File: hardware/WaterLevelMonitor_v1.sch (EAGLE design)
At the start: 38 parts, among them J1 D24V5F5, J2 AVR_SPI_PRG_6PTH, J5 D24V5F5, J6 D24V5F5, J7 RJ45, Q1 NDP6020P, Q4 2N3904, U1 ATMEGA328P_PDIP

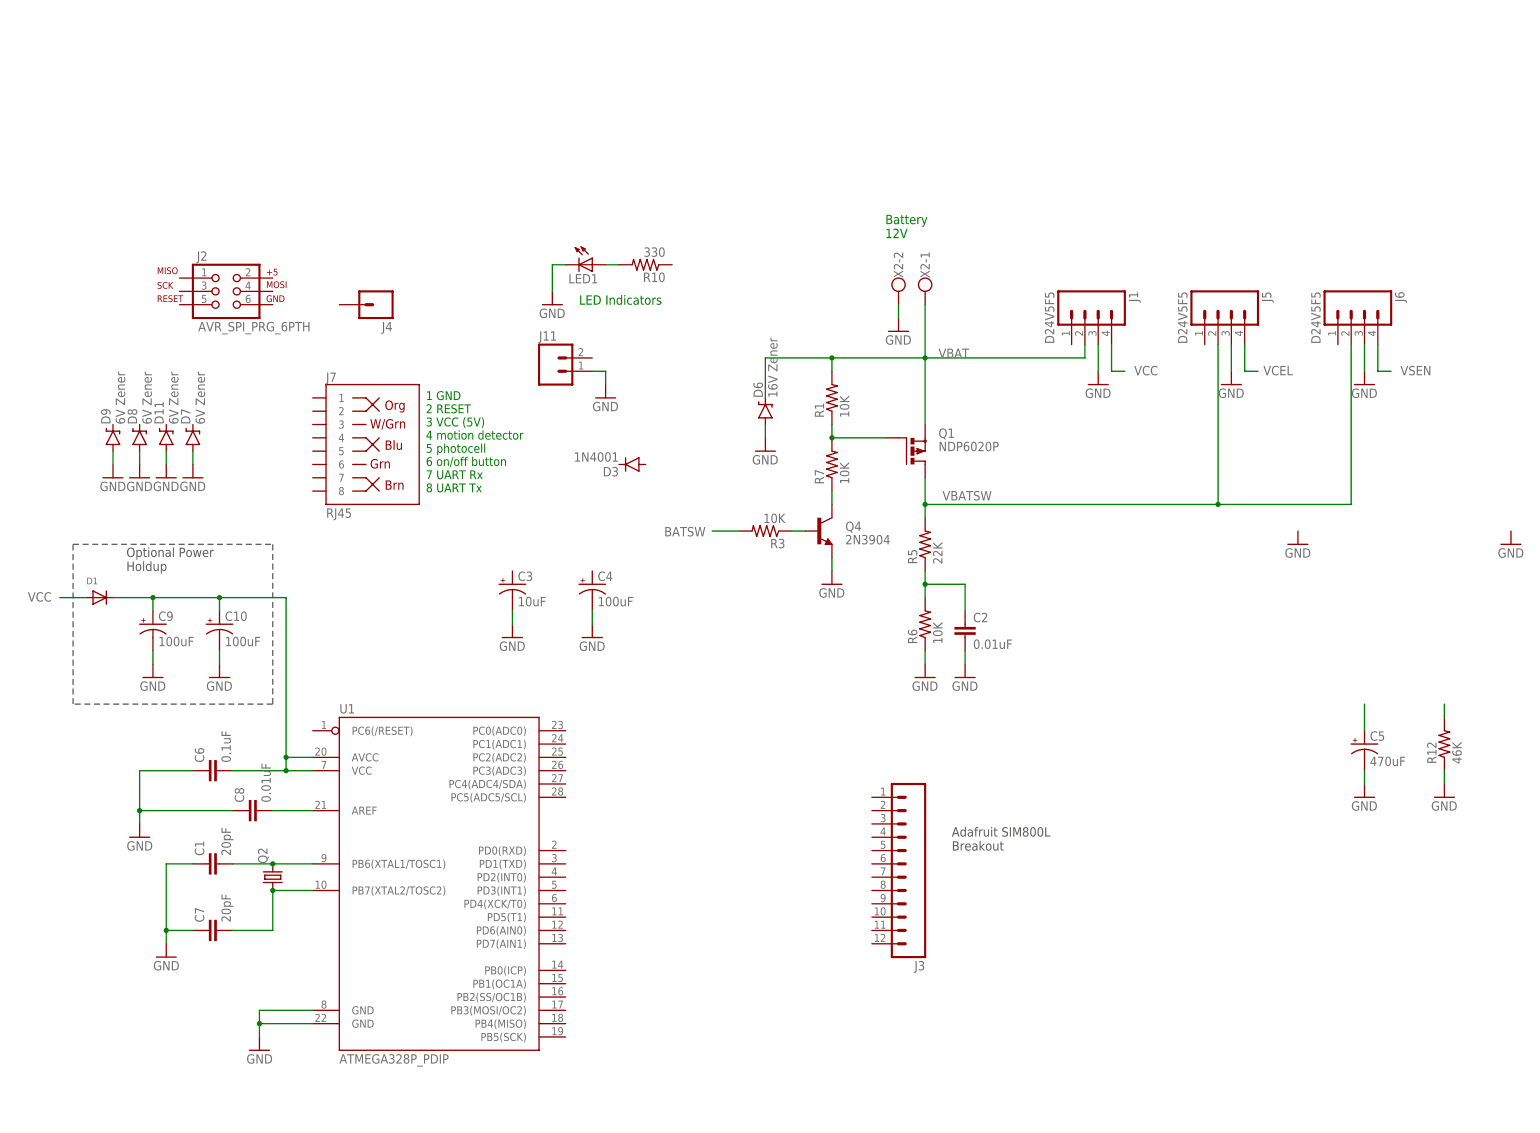
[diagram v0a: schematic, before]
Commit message: Add files via upload
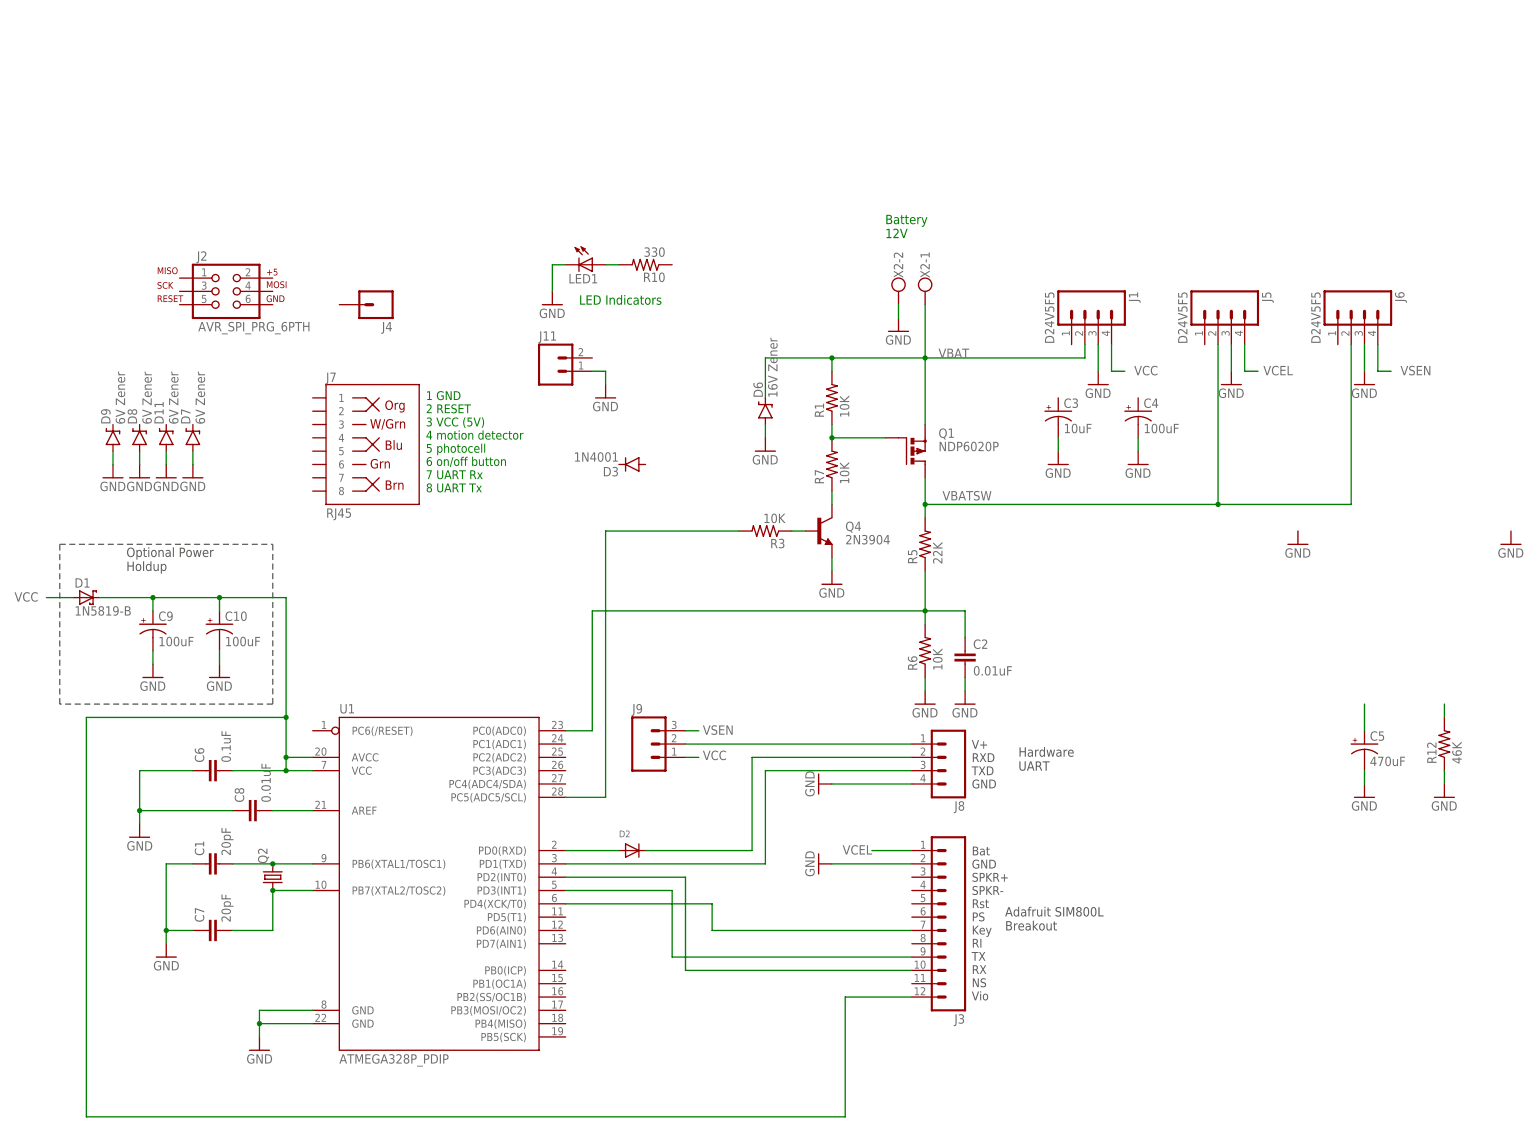
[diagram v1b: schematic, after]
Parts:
- added D2: (no value), adafruit:DIODEDO-1N4148
- added J8: (no value), SparkFun-Connectors:M04PTH
- added J9: (no value), SparkFun-Connectors:M03PTH
- D1: value (none) -> 1N5819-B; device adafruit:DIODEDO-1N4148 -> diode:1N5819-B
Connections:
- removed net BATSW: R3.2
- new net N$12: J3.7, U1.PD4(XCK/T0)
- new net N$13: D2.C, J8.2
- new net N$15: D2.A, U1.PD0(RXD)
- new net N$16: J3.9, U1.PD3(INT1)
- new net N$17: J3.10, U1.PD2(INT0)
- new net N$18: J8.1, J9.2
- new net N$19: R3.2, U1.PC5(ADC5/SCL)
- new net N$7: J8.3, U1.PD1(TXD)
- net GND: now also J3.2, J8.4
- net N$4: now also J3.12
- net N$6: now also U1.PC0(ADC0)
- net VCC: now also J9.1
- net VCEL: now also J3.1
- net VSEN: now also J9.3
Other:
- note added: "Bat GND SPKR+ SPKR- Rst PS Key RI TX RX NS Vio"
- note added: "Hardware UART"
- note added: "V+ RXD TXD GND"
- moved on the sheet: C2, C3, C4, J3, R6

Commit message: Add files via upload
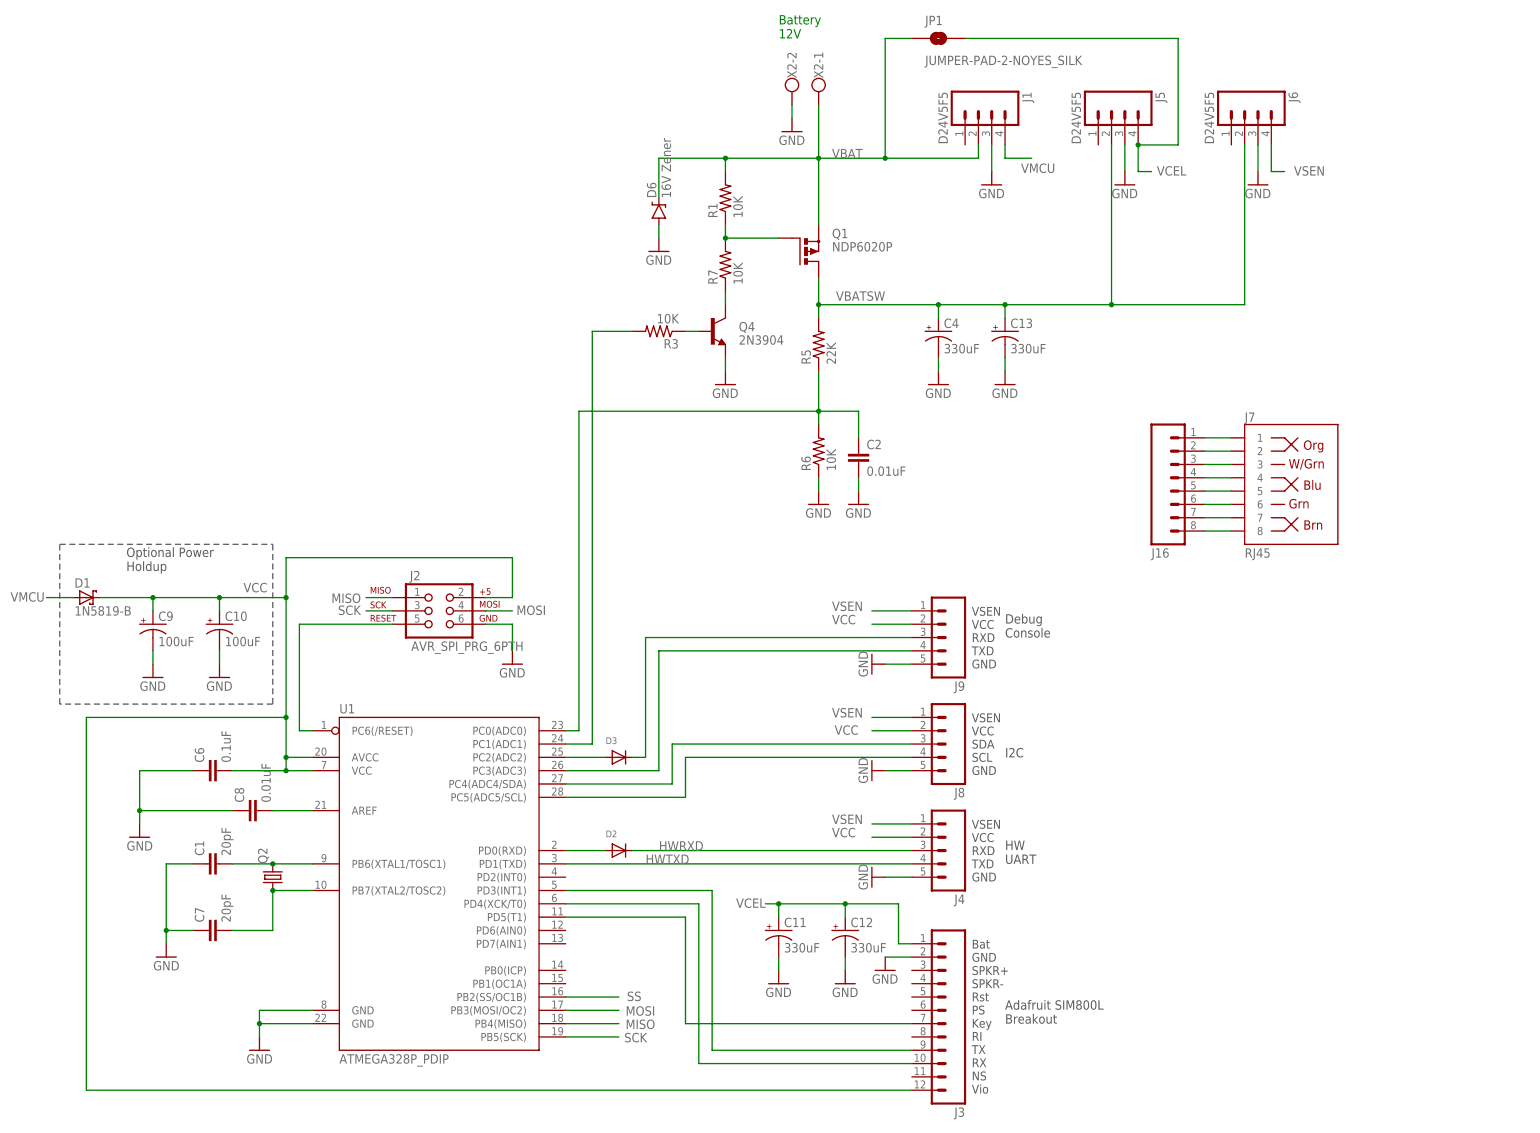
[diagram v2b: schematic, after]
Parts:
- removed C3: 10uF, SparkFun-Capacitors:CAP_POLPTH1
- removed C5: 470uF, SparkFun-Capacitors:CAP_POLPTH4
- removed D11, D7, D8, D9: 6V Zener, SparkFun-DiscreteSemi:DIODE-ZENERPTH
- removed J11: (no value), SparkFun-Connectors:M02PTH
- removed LED1: (no value), adafruit:LED5MM
- removed R10: 330, resistor:R-US_0204/5
- removed R12: 46K, resistor:R-US_0204/5
- added C11, C12, C13: 330uF, SparkFun-Capacitors:CAP_POLPTH1
- added J16: (no value), SparkFun-Connectors:M08SILK_FEMALE_PTH
- added JP1: JUMPER-PAD-2-NOYES_SILK, SparkFun-Passives:JUMPER-PAD-2-NOYES_SILK
- C4: value 100uF -> 330uF
- D3: value 1N4001 -> (none); device SparkFun-DiscreteSemi:DIODEPTH -> adafruit:DIODEDO-1N4148
- J4: device SparkFun-Connectors:M01PTH -> SparkFun-Connectors:M05PTH
- J8: device SparkFun-Connectors:M04PTH -> SparkFun-Connectors:M05PTH
- J9: device SparkFun-Connectors:M03PTH -> SparkFun-Connectors:M05PTH
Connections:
- removed net N$12: J3.7, U1.PD4(XCK/T0)
- removed net N$13: D2.C, J8.2
- removed net N$17: J3.10, U1.PD2(INT0)
- removed net N$18: J8.1, J9.2
- removed net N$4 (its old number): C10.+, C6.2, C9.+, D1.C, J3.12, U1.AVCC, U1.VCC
- removed net N$7: J8.3, U1.PD1(TXD)
- removed net N$8: C5.+
- new net HWRXD: D2.C, J4.3
- new net HWTXD: J4.4, U1.PD1(TXD)
- new net MISO: J2.1, U1.PB4(MISO)
- new net MOSI: J2.4, U1.PB3(MOSI/OC2)
- new net N$20: D3.A, U1.PC2(ADC2)
- new net N$21: D3.C, J9.3
- new net N$22: J9.4, U1.PC3(ADC3)
- new net N$25: J8.3, U1.PC4(ADC4/SDA)
- new net N$26: J8.4, U1.PC5(ADC5/SCL)
- new net N$27: J16.1, J7.1
- new net N$28: J16.2, J7.2
- new net N$29: J16.3, J7.3
- new net N$30: J16.4, J7.4
- new net N$31: J16.5, J7.5
- new net N$32: J2.5, U1.PC6(/RESET)
- new net N$33: J16.6, J7.6
- new net N$34: J16.7, J7.7
- new net N$35: J16.8, J7.8
- new net SCK: J2.3, U1.PB5(SCK)
- new net SS: U1.PB2(SS/OC1B)
- new net VMCU: D1.A, J1.4
- net GND: now also C11.-, C12.-, C13.-, J2.6, J4.5, J8.5, J9.5; no longer C3.-, C5.-, D11.A, D7.A, D8.A, D9.A, J11.1, J8.4, LED1.C, R12.1
- net N$1: now also J3.7, U1.PD5(T1); no longer LED1.A, R10.2
- net N$19: now also U1.PC1(ADC1); no longer U1.PC5(ADC5/SCL)
- net N$5: now also J3.10, U1.PD4(XCK/T0); no longer R12.2
- net VBAT: now also JP1.1
- net VBATSW: now also C13.+, C4.+
- net VCC: now also C10.+, C6.2, C9.+, D1.C, J2.2, J3.12, J4.2, J8.2, J9.2, U1.AVCC, U1.VCC; no longer D1.A, J1.4, J9.1
- net VCEL: now also C11.+, C12.+, JP1.2
- net VSEN: now also J4.1, J8.1, J9.1; no longer J9.3
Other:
- note added: "Debug Console"
- note added: "HW UART"
- note added: "I2C"
- note added: "VSEN VCC RXD TXD GND"
- note added: "VSEN VCC SDA SCL GND"
- note removed: "1 GND 2 RESET 3 VCC (5V) 4 motion detector 5 photocell 6 on/off button 7 UART Rx 8 UART Tx"
- note removed: "Hardware UART"
- note removed: "LED Indicators"
- note removed: "V+ RXD TXD GND"
- moved on the sheet: C2, C4, D2, D6, J1, J2, J3, J5, J6, J7, Q1, Q4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
